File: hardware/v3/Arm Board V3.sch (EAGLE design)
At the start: 66 parts, among them CN1 1X4-BIG, IC1 L6208D, IC2 L6208D, IC3 L6208D, IC4 7812TV, IC5 7812TV, Q3 Q_LTC490, U1 MAX3468CPA, U2 XBEE-1B3

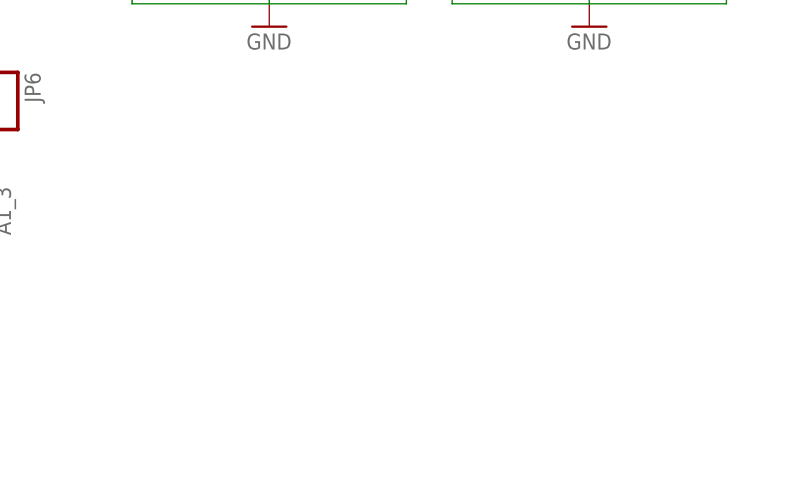
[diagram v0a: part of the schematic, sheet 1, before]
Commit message: 3V3 Vreg
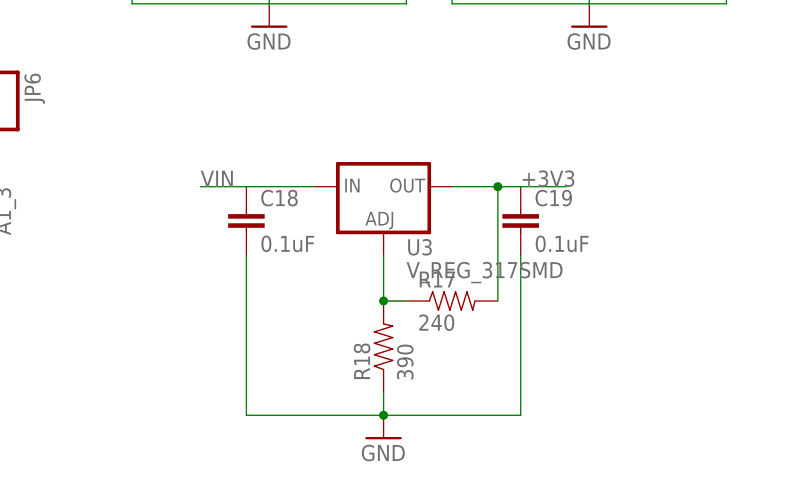
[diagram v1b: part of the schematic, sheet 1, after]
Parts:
- added C18, C19: 0.1uF, SparkFun-Capacitors:0.1UF-25V(+80/-20%)(0603)
- added R17: 240, SparkFun-Resistors:RESISTOR0805-RES
- added R18: 390, SparkFun-Resistors:RESISTOR0805-RES
- added U3: V_REG_317SMD, SparkFun-PowerIC:V_REG_317SMD
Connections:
- new net N$12: R17.1, R18.2, U3.ADJ
- net +3V3: now also C19.1, R17.2, U3.OUT
- net GND: now also C18.2, C19.2, R18.1
- net VIN: now also C18.1, U3.IN
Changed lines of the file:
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@@
 <part name="C15" library="SparkFun-Capacitors" deviceset="0.1UF-25V(+80/-20%)(0603)" device="" value="0.1uF"/>
 <part name="C17" library="SparkFun-Capacitors" deviceset="0.1UF-25V(+80/-20%)(0603)" device="" value="0.1uF"/>
+<part name="U3" library="SparkFun-PowerIC" deviceset="V_REG_317" device="SMD"/>
+<part name="GND20" library="SparkFun-Aesthetics" deviceset="GND" device=""/>
+<part name="R17" library="SparkFun-Resistors" deviceset="RESISTOR" device="0805-RES" value="240"/>
+<part name="R18" library="SparkFun-Resistors" deviceset="RESISTOR" device="0805-RES" value="390"/>
+<part name="C18" library="SparkFun-Capacitors" deviceset="0.1UF-25V(+80/-20%)(0603)" device="" value="0.1uF"/>
+<part name="C19" library="SparkFun-Capacitors" deviceset="0.1UF-25V(+80/-20%)(0603)" device="" value="0.1uF"/>
 </parts>
 <sheets>
@@
 <instance part="C15" gate="G$1" x="104.14" y="33.02"/>
 <instance part="C17" gate="G$1" x="109.22" y="33.02"/>
+<instance part="U3" gate="G$1" x="101.6" y="7.62"/>
+<instance part="GND20" gate="1" x="101.6" y="-20.32"/>
+<instance part="R17" gate="G$1" x="109.22" y="-5.08"/>
+<instance part="R18" gate="G$1" x="101.6" y="-10.16" rot="R90"/>
+<instance part="C18" gate="G$1" x="86.36" y="2.54"/>
+<instance part="C19" gate="G$1" x="116.84" y="2.54"/>
 </instances>
 <busses>
@@
 <pinref part="C17" gate="G$1" pin="2"/>
 </segment>
+<segment>
+<pinref part="GND20" gate="1" pin="GND"/>
+<pinref part="R18" gate="G$1" pin="1"/>
+<wire x1="101.6" y1="-15.24" x2="101.6" y2="-17.78" width="0.1524" layer="91"/>
+<pinref part="C19" gate="G$1" pin="2"/>
+<wire x1="116.84" y1="0" x2="116.84" y2="-17.78" width="0.1524" layer="91"/>
+<wire x1="116.84" y1="-17.78" x2="101.6" y2="-17.78" width="0.1524" layer="91"/>
+<pinref part="C18" gate="G$1" pin="2"/>
+<wire x1="101.6" y1="-17.78" x2="86.36" y2="-17.78" width="0.1524" layer="91"/>
+<wire x1="86.36" y1="-17.78" x2="86.36" y2="0" width="0.1524" layer="91"/>
+<junction x="101.6" y="-17.78"/>
+</segment>
 </net>
 <net name="A1_1" class="0">
@@
 <pinref part="C17" gate="G$1" pin="1"/>
 </segment>
+<segment>
+<pinref part="U3" gate="G$1" pin="IN"/>
+<pinref part="C18" gate="G$1" pin="1"/>
+<wire x1="86.36" y1="7.62" x2="93.98" y2="7.62" width="0.1524" layer="91"/>
+<wire x1="86.36" y1="7.62" x2="81.28" y2="7.62" width="0.1524" layer="91"/>
+<label x="81.28" y="7.62" size="1.778" layer="95"/>
+</segment>
 </net>
 <net name="A1_3" class="0">
@@
 </segment>
 </net>
+<net name="N$12" class="0">
+<segment>
+<pinref part="U3" gate="G$1" pin="ADJ"/>
+<pinref part="R18" gate="G$1" pin="2"/>
+<wire x1="101.6" y1="-5.08" x2="101.6" y2="0" width="0.1524" layer="91"/>
+<pinref part="R17" gate="G$1" pin="1"/>
+<wire x1="104.14" y1="-5.08" x2="101.6" y2="-5.08" width="0.1524" layer="91"/>
+<junction x="101.6" y="-5.08"/>
+</segment>
+</net>
+<net name="+3V3" class="0">
+<segment>
+<pinref part="U3" gate="G$1" pin="OUT"/>
+<pinref part="C19" gate="G$1" pin="1"/>
+<wire x1="116.84" y1="7.62" x2="114.3" y2="7.62" width="0.1524" layer="91"/>
+<pinref part="R17" gate="G$1" pin="2"/>
+<wire x1="114.3" y1="7.62" x2="109.22" y2="7.62" width="0.1524" layer="91"/>
+<wire x1="114.3" y1="-5.08" x2="114.3" y2="7.62" width="0.1524" layer="91"/>
+<junction x="114.3" y="7.62"/>
+<wire x1="116.84" y1="7.62" x2="121.92" y2="7.62" width="0.1524" layer="91"/>
+<label x="116.84" y="7.62" size="1.778" layer="95"/>
+</segment>
+</net>
